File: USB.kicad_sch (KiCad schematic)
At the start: 34 parts, among them J1 USB_C_Receptable_USB2.0, U1 AP2141WG-7, U2 3V3

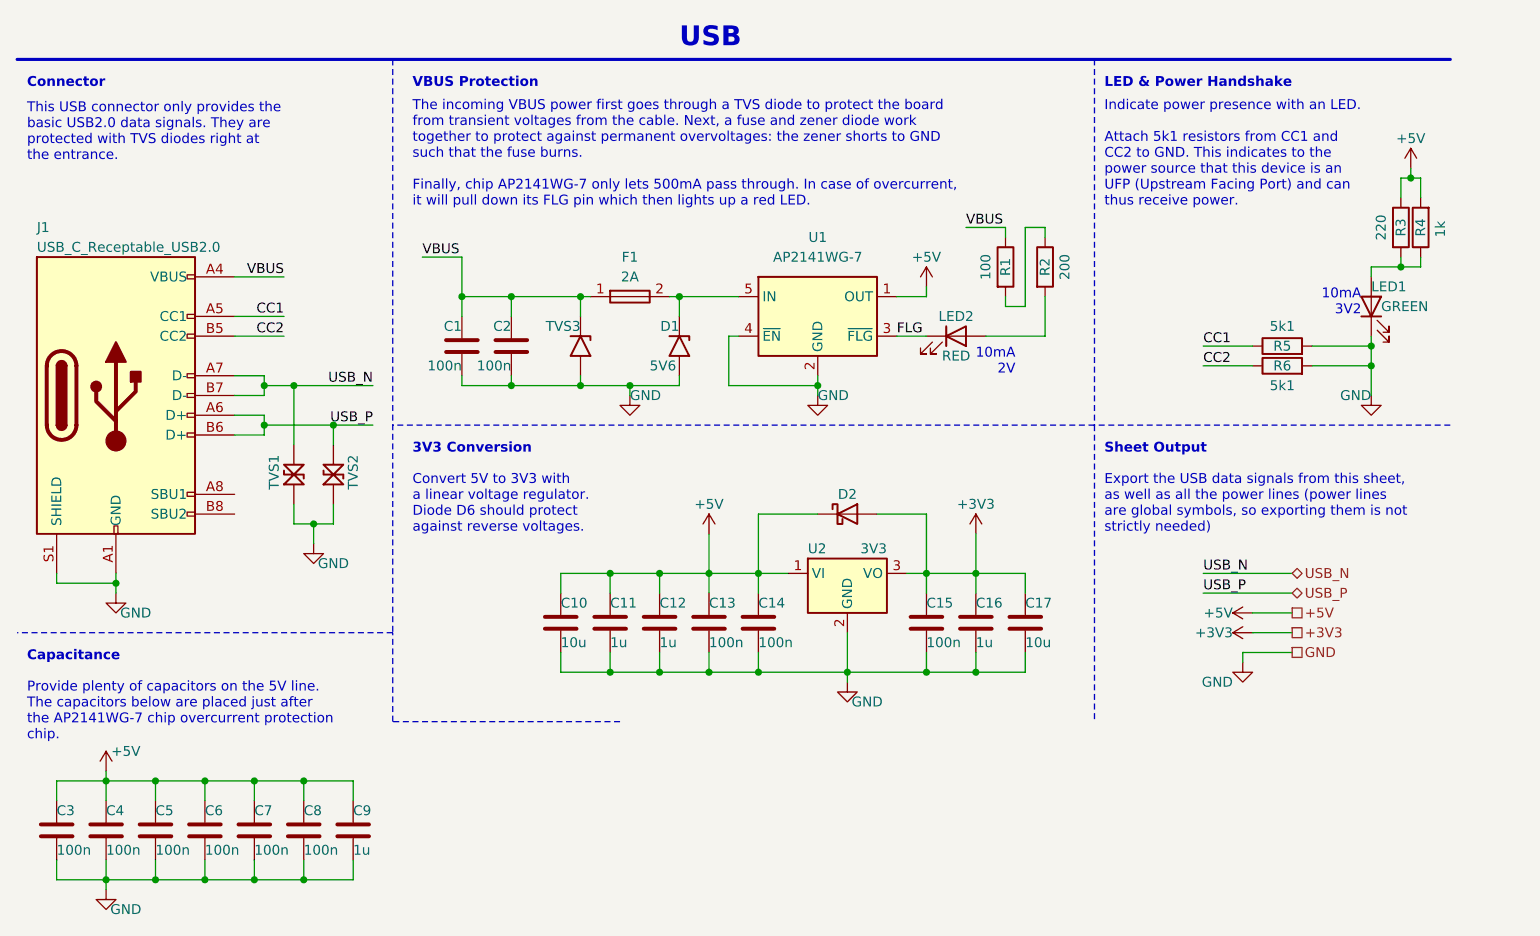
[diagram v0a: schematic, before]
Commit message: Apply suggestions from Petr Dvorak
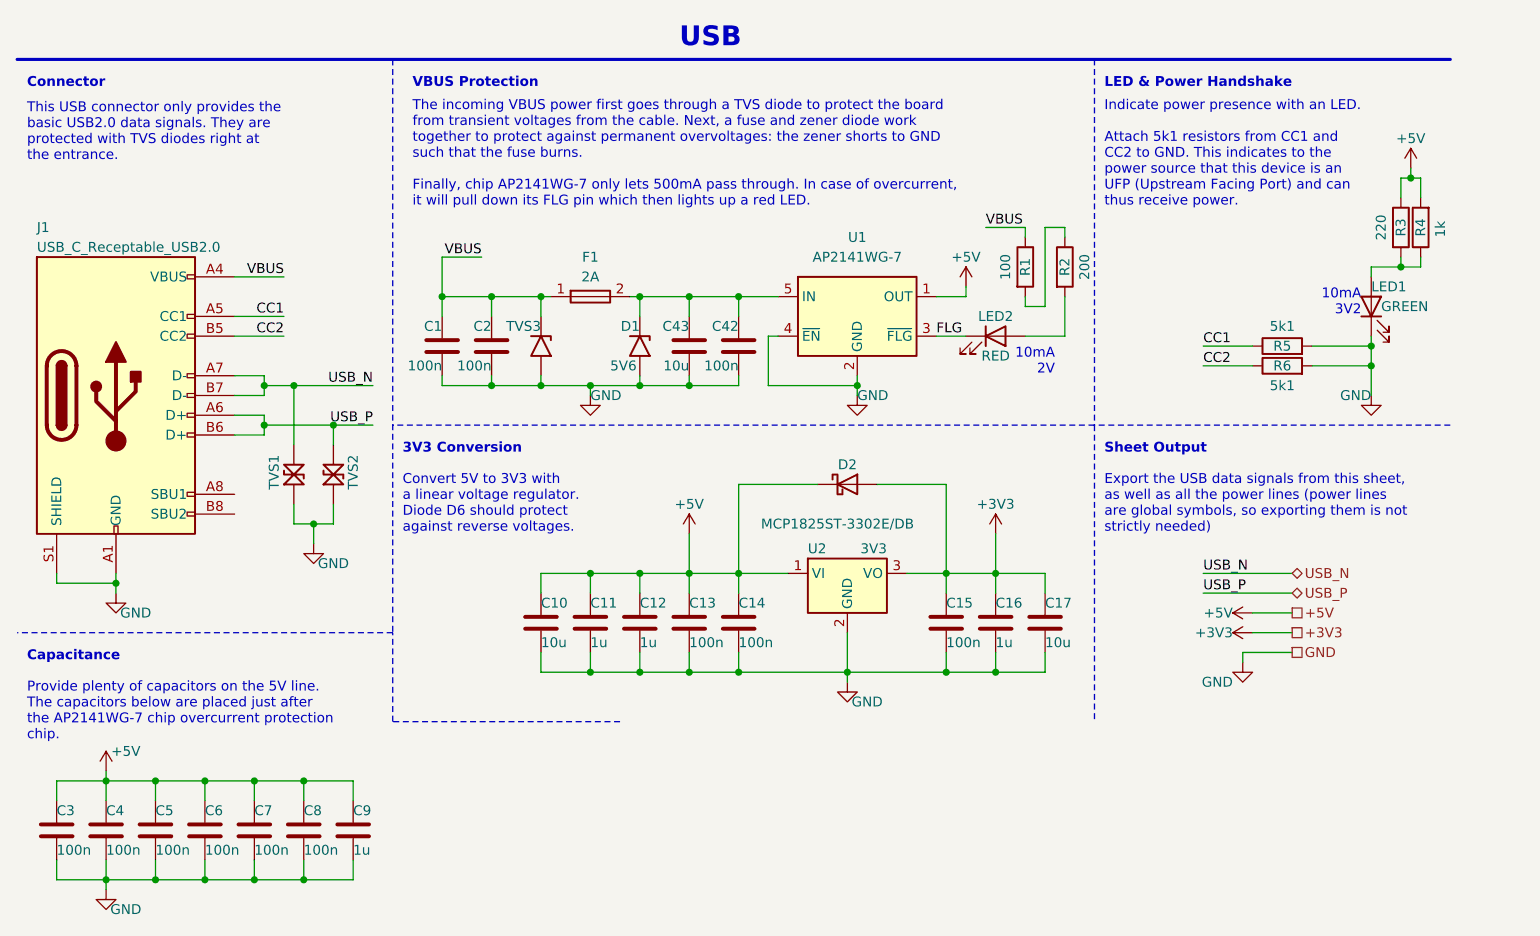
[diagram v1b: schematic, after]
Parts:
- added C42: 100n, Capacitor_SMD:C_0402_1005Metric_Pad0.74x0.62mm_HandSolder, symbol Device:C
- added C43: 10u, Capacitor_SMD:C_0805_2012Metric, symbol Device:C
- C1, C2: Comment 50V 100nF X7R ±10% 0402 Multilayer Ceramic Capacitors MLCC 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 -> 50V 100nF X7R ±10% 0402
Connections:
- net GND: now also C42.1, C43.2
- net at D1.1 (A1), F1.2, U1.5 (IN): now also C42.2, C43.1
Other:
- moved on the sheet: C1, C10, C11, C12, C13, C14, C15, C16, C17, C2, D1, D2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
